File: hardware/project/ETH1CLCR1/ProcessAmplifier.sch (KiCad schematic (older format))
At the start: 77 parts, among them U901 TL072, U902 TL072, U903 TL072, U904 TL072, U905 TL071, U906 TL071, U907 AQY212GS, U908 AQY212GS, U909 AQY212GS, U910 AQY212GS, U911 AQY212GS, U912 AQY212GS, U913 AQY212GS, U914 AQY212GS, U915 AQY212GS, U916 AQY212GS

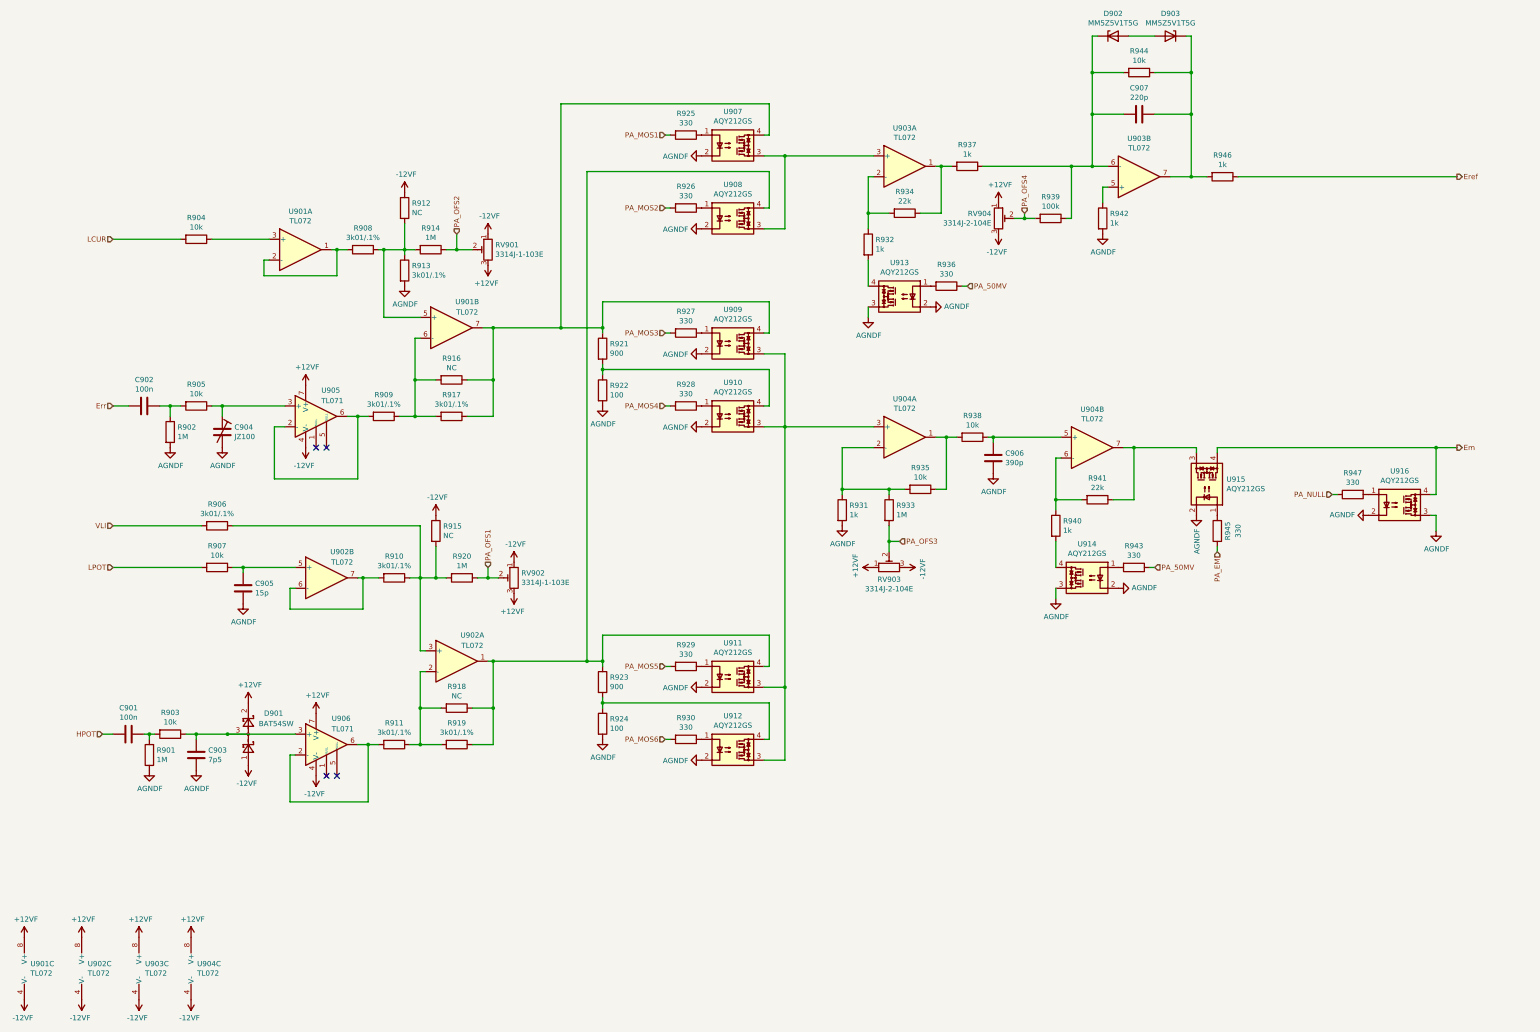
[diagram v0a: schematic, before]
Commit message: Changes in schematics.
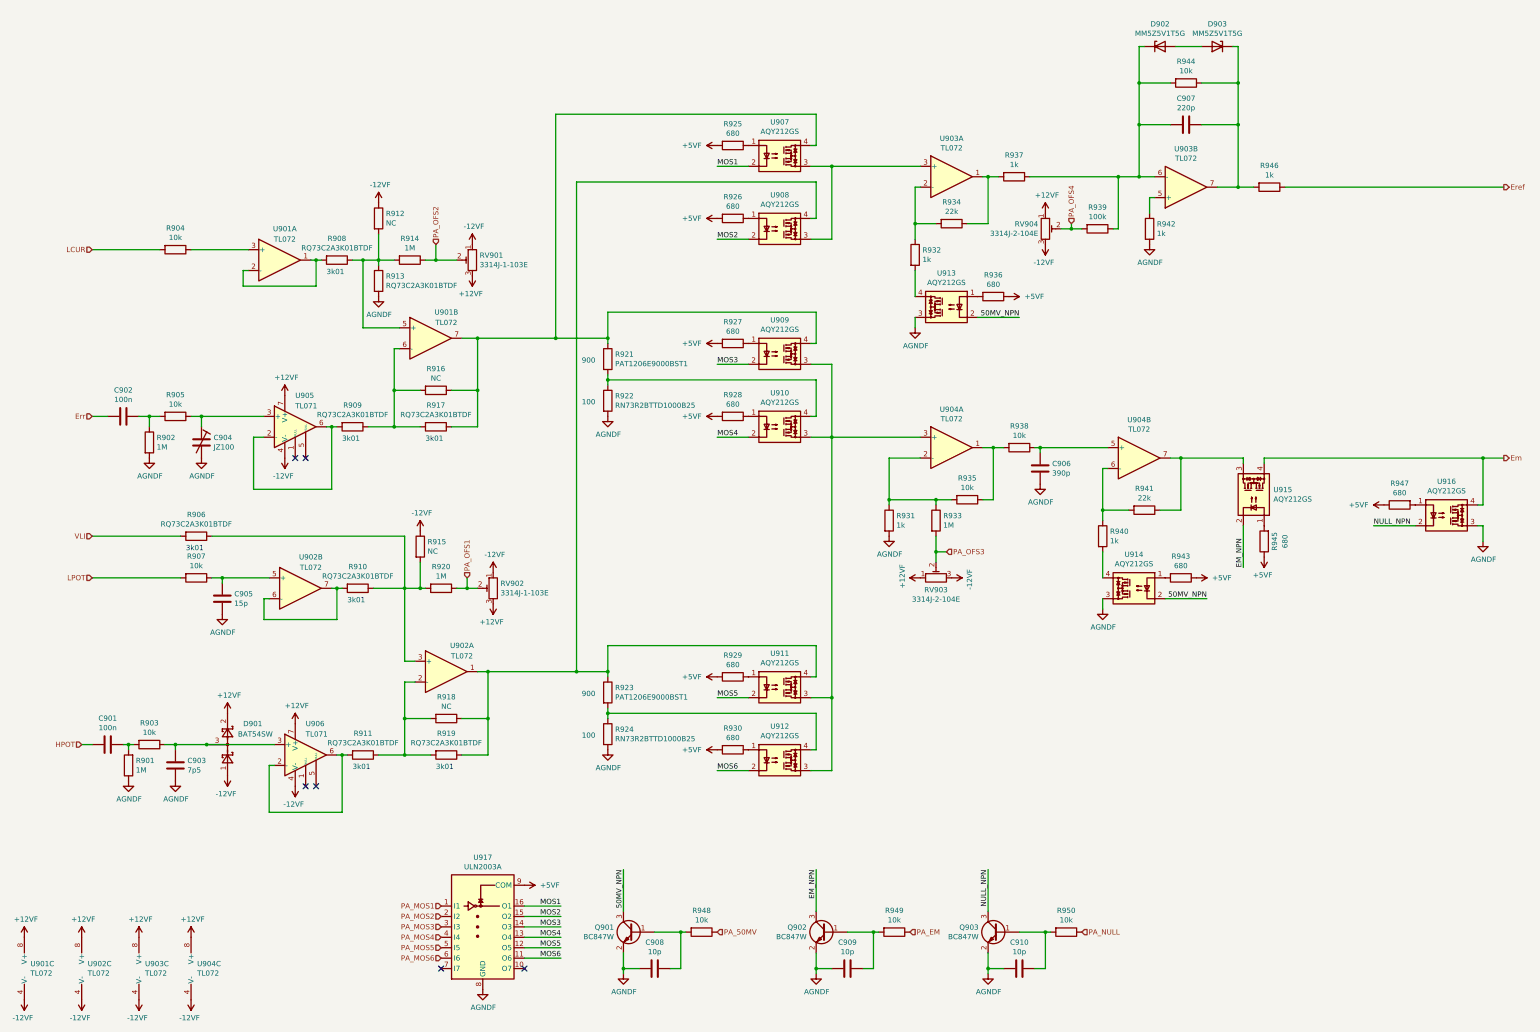
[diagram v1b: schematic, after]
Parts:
- added C908, C909, C910: 10p, Capacitor_SMD:C_0603_1608Metric_Pad1.05x0.95mm_HandSolder, symbol Device:C
- added Q901, Q902, Q903: BC847W, Package_TO_SOT_SMD:SOT-323_SC-70, symbol Transistor_BJT:BC847W
- added R948, R949, R950: 10k, Resistor_SMD:R_0603_1608Metric_Pad1.05x0.95mm_HandSolder, symbol Device:R
- added U917: ULN2003A, Package_SO:TSSOP-16_4.4x5mm_P0.65mm, symbol Transistor_Array:ULN2003A
- R906, R908, R909, R910, R911, R913, R917, R919: value 3k01/.1% -> RQ73C2A3K01BTDF; footprint Resistor_SMD:R_0603_1608Metric_Pad1.05x0.95mm_HandSolder -> Resistor_SMD:R_0805_2012Metric_Pad1.15x1.40mm_HandSolder
- R921, R923: value 900 -> PAT1206E9000BST1; footprint Resistor_SMD:R_0603_1608Metric_Pad1.05x0.95mm_HandSolder -> Resistor_SMD:R_1206_3216Metric_Pad1.42x1.75mm_HandSolder
- R922, R924: value 100 -> RN73R2BTTD1000B25; footprint Resistor_SMD:R_0603_1608Metric_Pad1.05x0.95mm_HandSolder -> Resistor_SMD:R_1206_3216Metric_Pad1.42x1.75mm_HandSolder
- R925, R926, R927, R928, R929, R930, R936, R943, R945, R947: value 330 -> 680
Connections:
- net AGNDF: now also C908.2, C909.2, C910.2, Q901.2 (E), Q902.2 (E), Q903.2 (E), U917.8 (GND); no longer U907.2, U908.2, U909.2, U910.2, U911.2, U912.2, U913.2, U914.2, U915.2, U916.2
- net PA_50MV: now also R948.1; no longer R936.1, R943.1
- net PA_EM: now also R949.1; no longer R945.1
- net PA_MOS1: now also U917.1 (I1); no longer R925.2
- net PA_MOS2: now also U917.2 (I2); no longer R926.2
- net PA_MOS3: now also U917.3 (I3); no longer R927.2
- net PA_MOS4: now also U917.4 (I4); no longer R928.2
- net PA_MOS5: now also U917.5 (I5); no longer R929.2
- net PA_MOS6: now also U917.6 (I6); no longer R930.2
- net PA_NULL: now also R950.1; no longer R947.1
- new net: C908.1, Q901.1 (B), R948.2
- new net: C909.1, Q902.1 (B), R949.2
- new net: C910.1, Q903.1 (B), R950.2
- new net +5VF: R925.2, R926.2, R927.2, R928.2, R929.2, R930.2, R936.1, R943.1, R945.1, R947.1, U917.9 (COM)
- new net 50MV_NPN: Q901.3 (C), U913.2, U914.2
- new net EM_NPN: Q902.3 (C), U915.2
- new net MOS1: U907.2, U917.16 (O1)
- new net MOS2: U908.2, U917.15 (O2)
- new net MOS3: U909.2, U917.14 (O3)
- new net MOS4: U910.2, U917.13 (O4)
- new net MOS5: U911.2, U917.12 (O5)
- new net MOS6: U912.2, U917.11 (O6)
- new net NULL_NPN: Q903.3 (C), U916.2
- no-connect marks 4 -> 6
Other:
- note added: "100"
- note added: "3k01"
- note added: "900"
- moved on the sheet: C901, C902, C903, C904, C905, C906, C907, D901, D902, D903, R901, R902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
